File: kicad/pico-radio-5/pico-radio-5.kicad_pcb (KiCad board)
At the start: 2 copper layers, 86.5 x 91.5 mm, 42 parts, among them J1 HF Amplifier, J2 MW/SW antenna, J3 FM antenna, J4 SW antenna, Q1 PN2222A, Q2 PN2222A, SW1 Reset, U1 SI4732-A10-GS, U2 TFT_320x240, U3 KY-040, Y1 32.762kHz

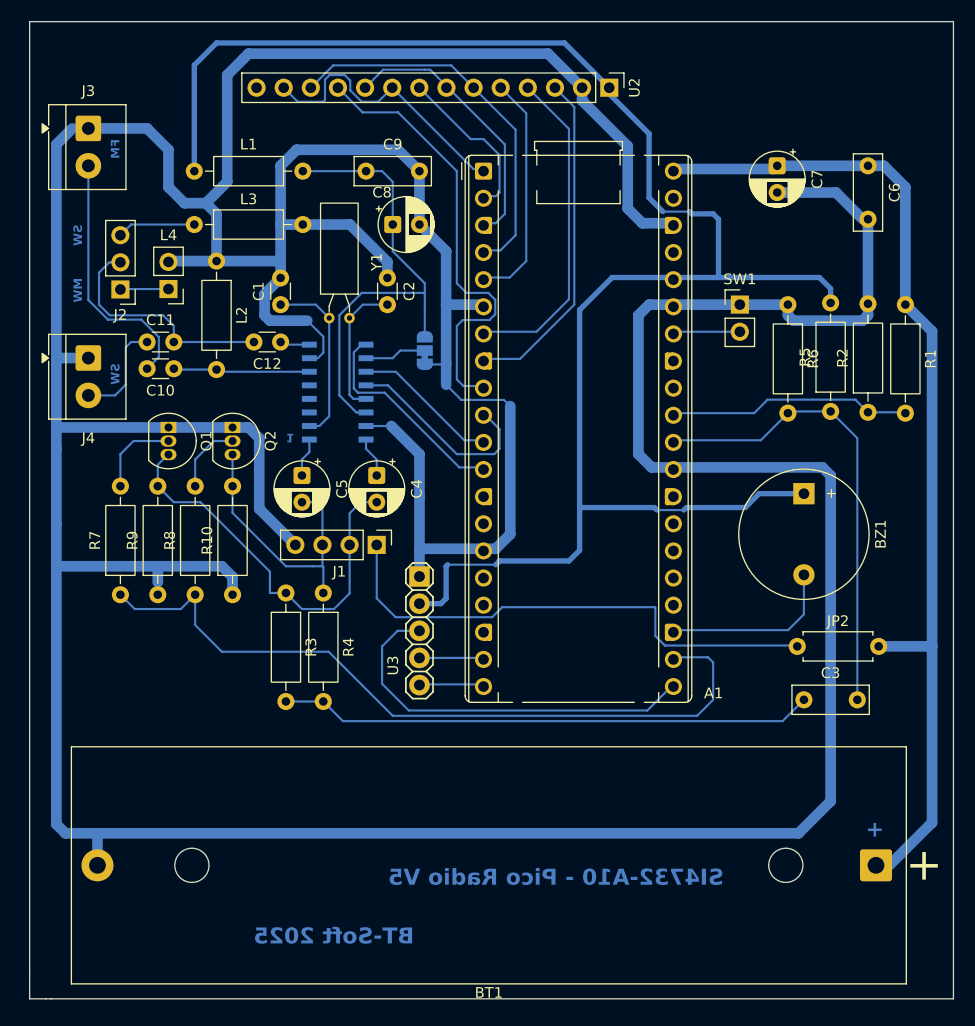
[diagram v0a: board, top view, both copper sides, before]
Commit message: Refactor code structure for improved readability and maintainability
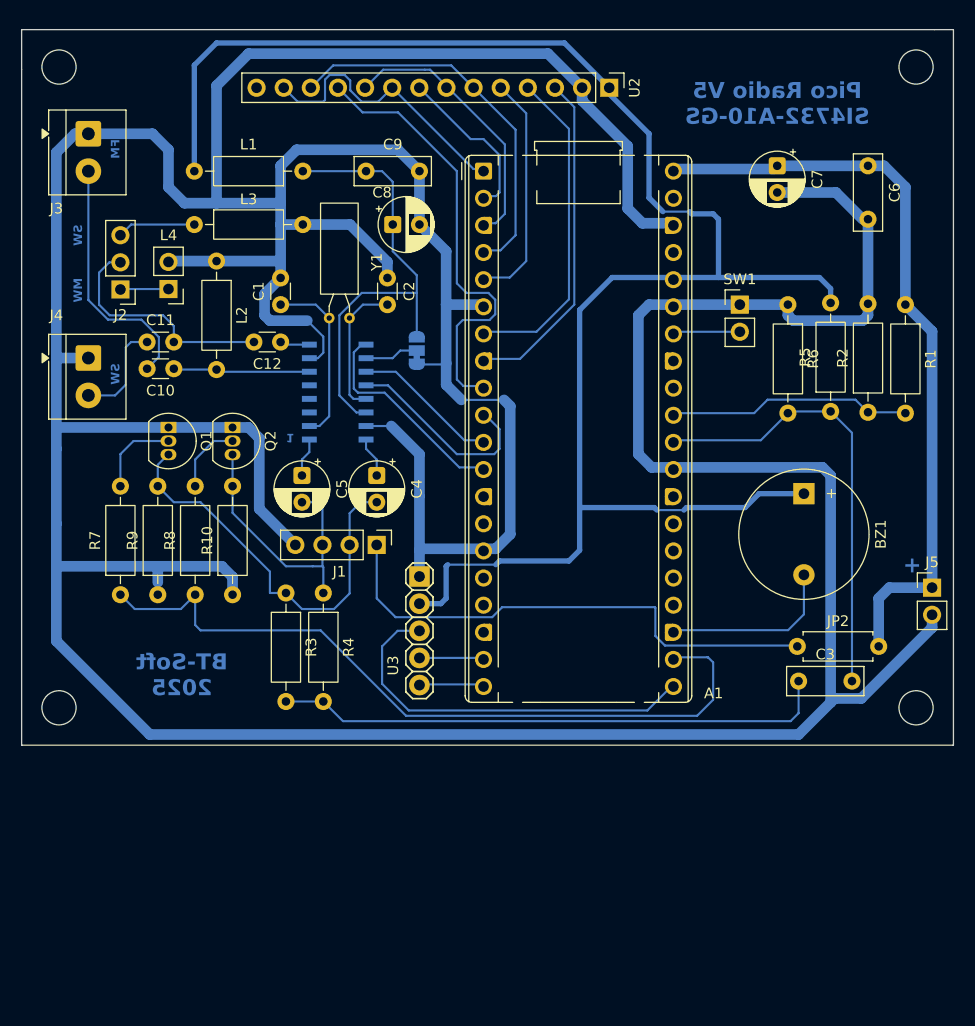
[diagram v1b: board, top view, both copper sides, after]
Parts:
- removed BT1: BK-18650-PC2, Battery:BatteryHolder_MPD_BK-18650-PC2
- added J5: Batterry, Connector_PinHeader_2.54mm:PinHeader_1x02_P2.54mm_Vertical, F.Cu at (114.0, 92.5)
- added REF**: MountingHole_3.2mm_M3, MountingHole:MountingHole_3.2mm_M3, F.Cu at (32.2, 43.8)
- added REF**: MountingHole_3.2mm_M3, MountingHole:MountingHole_3.2mm_M3, F.Cu at (112.5, 43.8)
- added REF**: MountingHole_3.2mm_M3, MountingHole:MountingHole_3.2mm_M3, F.Cu at (32.2, 103.8)
- added REF**: MountingHole_3.2mm_M3, MountingHole:MountingHole_3.2mm_M3, F.Cu at (112.5, 103.8)
- moved C3 1.82 mm to (101.5, 101.2)
- moved JP1 0.75 mm to (65.8, 70.3)
- moved J3 0.50 mm to (35.0, 50.0)
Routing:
- net +Vbus: track 95.1 -> 71.1 mm
- net GND: track 527.1 -> 514.6 mm
- net Net-(C3-Pad1): track 50.1 -> 52.1 mm
- net AD_FFT_AUDIO: track 43.9 -> 41.9 mm
- net Net-(JP1-B): track 44.1 -> 43.0 mm
- net Net-(JP1-C): track 5.80 -> 5.05 mm
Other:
- board size 86.5 x 91.5 mm -> 87.2 x 67 mm
- board text added: "Pico Radio V5 SI4732-A10-GS"
- board text removed: "SI4732-A10 - Pico Radio V5"
